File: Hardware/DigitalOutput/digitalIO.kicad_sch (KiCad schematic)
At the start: 0 parts

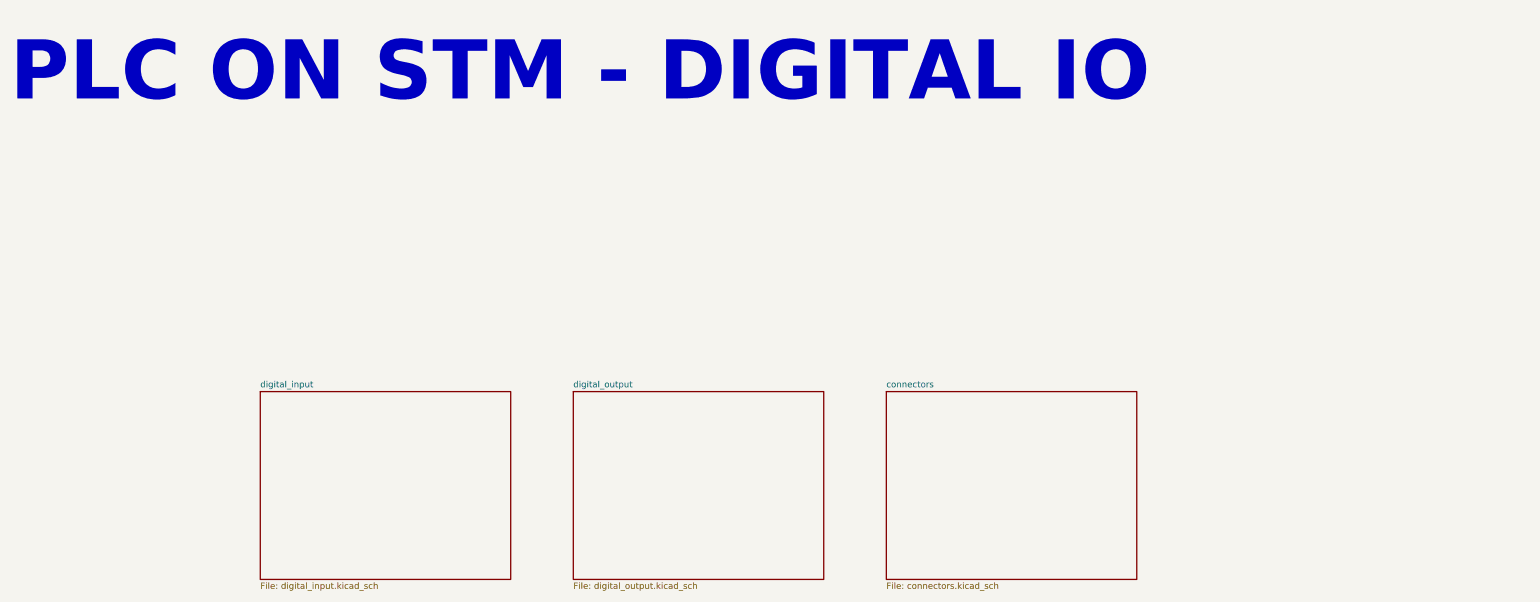
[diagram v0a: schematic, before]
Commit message: schematic update & pcb update
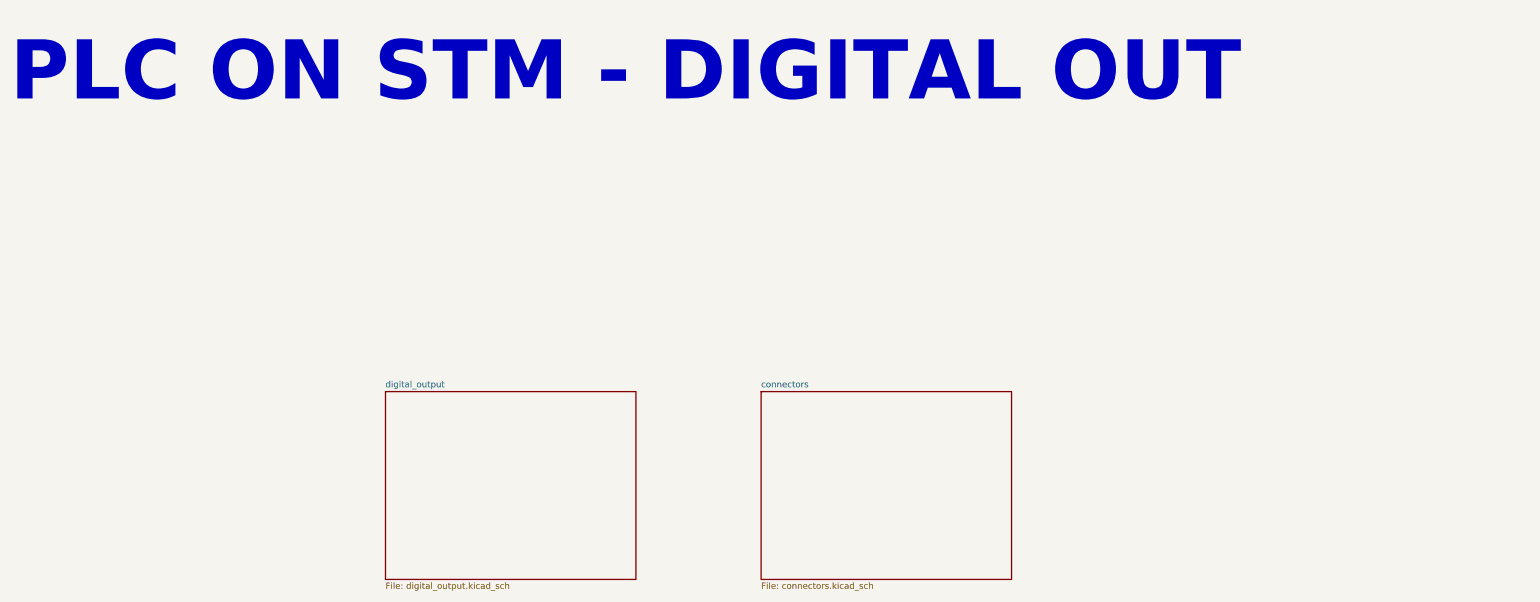
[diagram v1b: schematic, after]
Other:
- removed sheet digital_input
- note added: "PLC ON STM - DIGITAL OUT"
- note removed: "PLC ON STM - DIGITAL IO"
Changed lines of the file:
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@@
 		(company "Author: Grzegorz Potocki")
 	)
-	(text "PLC ON STM - DIGITAL IO"
+	(text "PLC ON STM - DIGITAL OUT"
 		(exclude_from_sim no)
 		(at 12.7 24.13 0)
@@
 	)
 	(sheet
-		(at 127 88.9)
+		(at 88.9 88.9)
 		(size 50.8 38.1)
 		(exclude_from_sim no)
@@
 		)
 		(property "Sheetname" "digital_output"
-			(at 127 88.1884 0)
+			(at 88.9 88.1884 0)
 			(effects
 				(font
@@
 		)
 		(property "Sheetfile" "digital_output.kicad_sch"
-			(at 127 127.5846 0)
+			(at 88.9 127.5846 0)
 			(effects
 				(font
@@
 	)
 	(sheet
-		(at 190.5 88.9)
+		(at 165.1 88.9)
 		(size 50.8 38.1)
 		(exclude_from_sim no)
@@
 		)
 		(property "Sheetname" "connectors"
-			(at 190.5 88.1884 0)
+			(at 165.1 88.1884 0)
 			(effects
 				(font
@@
 		)
 		(property "Sheetfile" "connectors.kicad_sch"
-			(at 190.5 127.5846 0)
+			(at 165.1 127.5846 0)
 			(effects
 				(font
@@
 				)
 			)
-		)
-	)
-	(sheet
-		(at 63.5 88.9)
-		(size 50.8 38.1)
-		(exclude_from_sim no)
-		(in_bom yes)
-		(on_board yes)
-		(dnp no)
-		(fields_autoplaced yes)
-		(stroke
-			(width 0.1524)
-			(type solid)
-		)
-		(fill
-			(color 0 0 0 0.0000)
-		)
-		(property "Sheetname" "digital_input"
-			(at 63.5 88.1884 0)
-			(effects
-				(font
-					(size 1.27 1.27)
-				)
-				(justify left bottom)
-			)
-		)
-		(property "Sheetfile" "digital_input.kicad_sch"
-			(at 63.5 127.5846 0)
-			(effects
-				(font
-					(size 1.27 1.27)
-				)
-				(justify left top)
-			)
-		)
-		(instances
-			(project "digitalIO"
-				(path "/b652b05a-4e3d-4ad1-b032-18886abe7d45"
-					(page "2")
-				)
-			)
